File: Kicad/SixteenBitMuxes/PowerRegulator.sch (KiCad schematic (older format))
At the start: 11 parts, among them J5 PowerTest_PinHeader, J6 9V Power JST XH, U1 AMS1117-5.0, U2 AMS1117-3.3

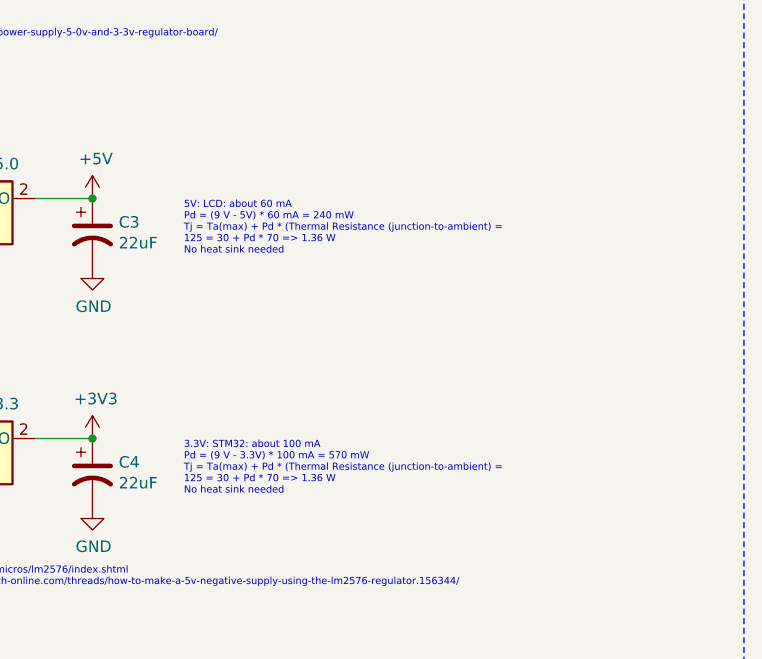
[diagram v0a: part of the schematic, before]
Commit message: PCB mostly
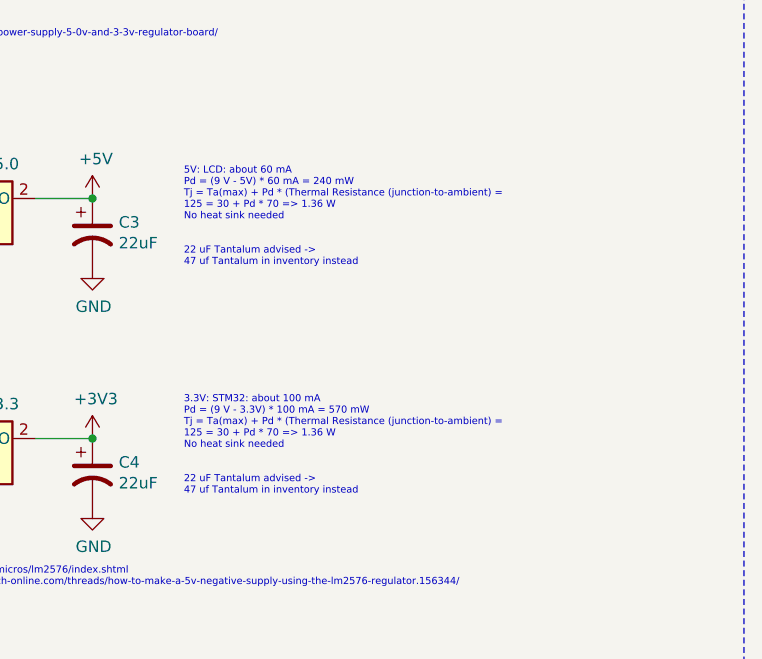
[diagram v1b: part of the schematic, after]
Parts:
- C3, C4: footprint Capacitor_THT:CP_Radial_D5.0mm_P2.50mm -> Diode_SMD:D_SMB_Handsoldering
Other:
- note added: "22 uF Tantalum advised ->\n47 uf Tantalum in inventory instead"
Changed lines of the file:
@@
 Text Notes 3250 2300 0    20   ~ 0
 9 mA, 81 mW
-Text Notes 4950 2050 0    31   ~ 0
+Text Notes 4950 1900 0    31   ~ 0
 5V: LCD: about 60 mA\nPd = (9 V - 5V) * 60 mA = 240 mW\nTj = Ta(max) + Pd * (Thermal Resistance (junction-to-ambient) =\n125 = 30 + Pd * 70 => 1.36 W\nNo heat sink needed
-Text Notes 4950 3100 0    31   ~ 0
+Text Notes 4950 2900 0    31   ~ 0
 3.3V: STM32: about 100 mA \nPd = (9 V - 3.3V) * 100 mA = 570 mW\nTj = Ta(max) + Pd * (Thermal Resistance (junction-to-ambient) =\n125 = 30 + Pd * 70 => 1.36 W\nNo heat sink needed
 Connection ~ 3550 2850
@@
 F 0 "C4" H 4665 3046 50  0000 L CNN
 F 1 "22uF" H 4665 2955 50  0000 L CNN
-F 2 "Capacitor_THT:CP_Radial_D5.0mm_P2.50mm" H 4550 3000 50  0001 C CNN
+F 2 "Diode_SMD:D_SMB_Handsoldering" H 4550 3000 50  0001 C CNN
 F 3 "~" H 4550 3000 50  0001 C CNN
 	1    4550 3000
@@
 F 0 "C3" H 4665 1996 50  0000 L CNN
 F 1 "22uF" H 4665 1905 50  0000 L CNN
-F 2 "Capacitor_THT:CP_Radial_D5.0mm_P2.50mm" H 4550 1950 50  0001 C CNN
+F 2 "Diode_SMD:D_SMB_Handsoldering" H 4550 1950 50  0001 C CNN
 F 3 "~" H 4550 1950 50  0001 C CNN
 	1    4550 1950
@@
 	1150 2300 1450 2300
 Connection ~ 1150 2300
+Text Notes 4950 2100 0    31   ~ 0
+22 uF Tantalum advised ->\n47 uf Tantalum in inventory instead
+Text Notes 4950 3100 0    31   ~ 0
+22 uF Tantalum advised ->\n47 uf Tantalum in inventory instead
 $EndSCHEMATC
